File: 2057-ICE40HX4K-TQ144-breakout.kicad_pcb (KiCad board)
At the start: 4 copper layers, 99.1 x 66 mm, 75 parts, among them J1 Conn_02x30_Odd_Even, J2 Conn_02x30_Odd_Even, J3 RaspberryPI-B+header, J4 USB4105-GF-A, J5 RaspberryPI-B+header, J6 Conn_02x08_Odd_Even, J7 Conn_02x01, J8 Micro_SD_Card_Det, U1 ICE40HX4K-TQ144, U2 AZ1117CH-3.3TRG1, U3 AZ1117CH-1.2, U4 AT45DB161D-SU, Y1 XLH536025_000000I

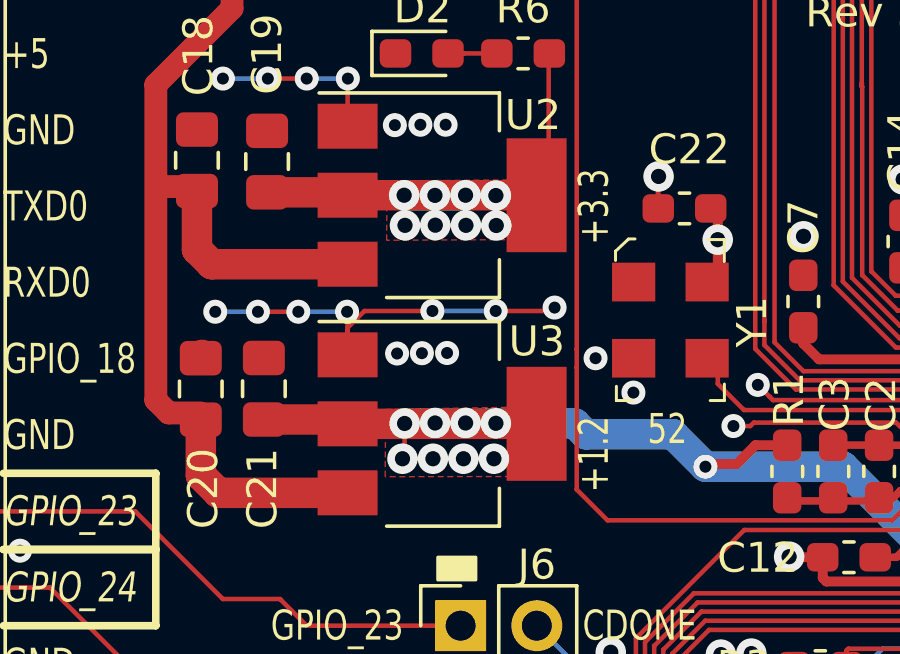
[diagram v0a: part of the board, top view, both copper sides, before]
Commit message: Fix power vias
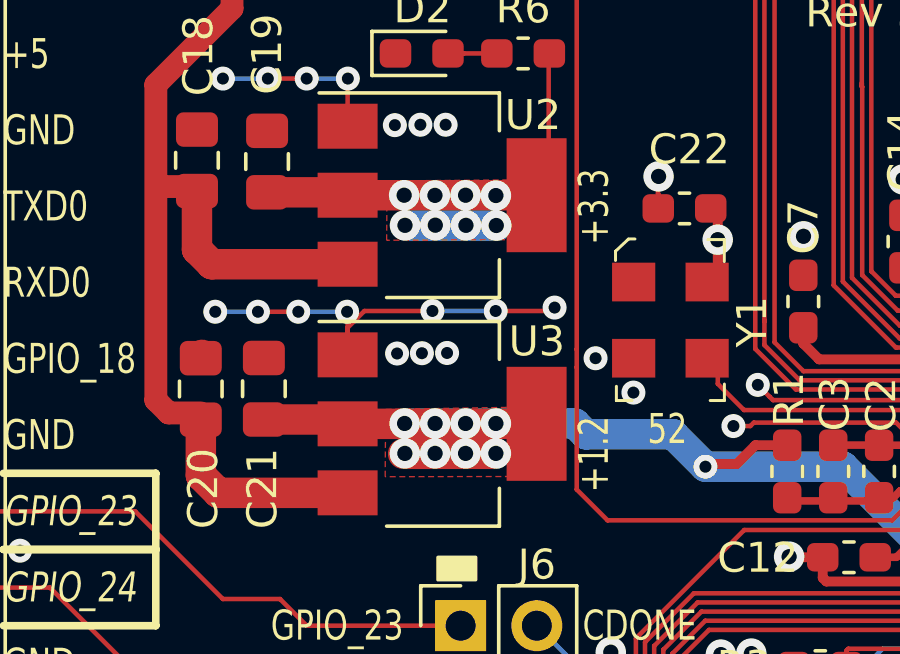
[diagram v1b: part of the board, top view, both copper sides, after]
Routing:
- net +3V3: track 103.8 -> 107.9 mm
- net +1V2: track 123.6 -> 125.4 mm
